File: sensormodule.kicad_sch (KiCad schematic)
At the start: 21 parts, among them X1 32.768KHz, X2 16MHz

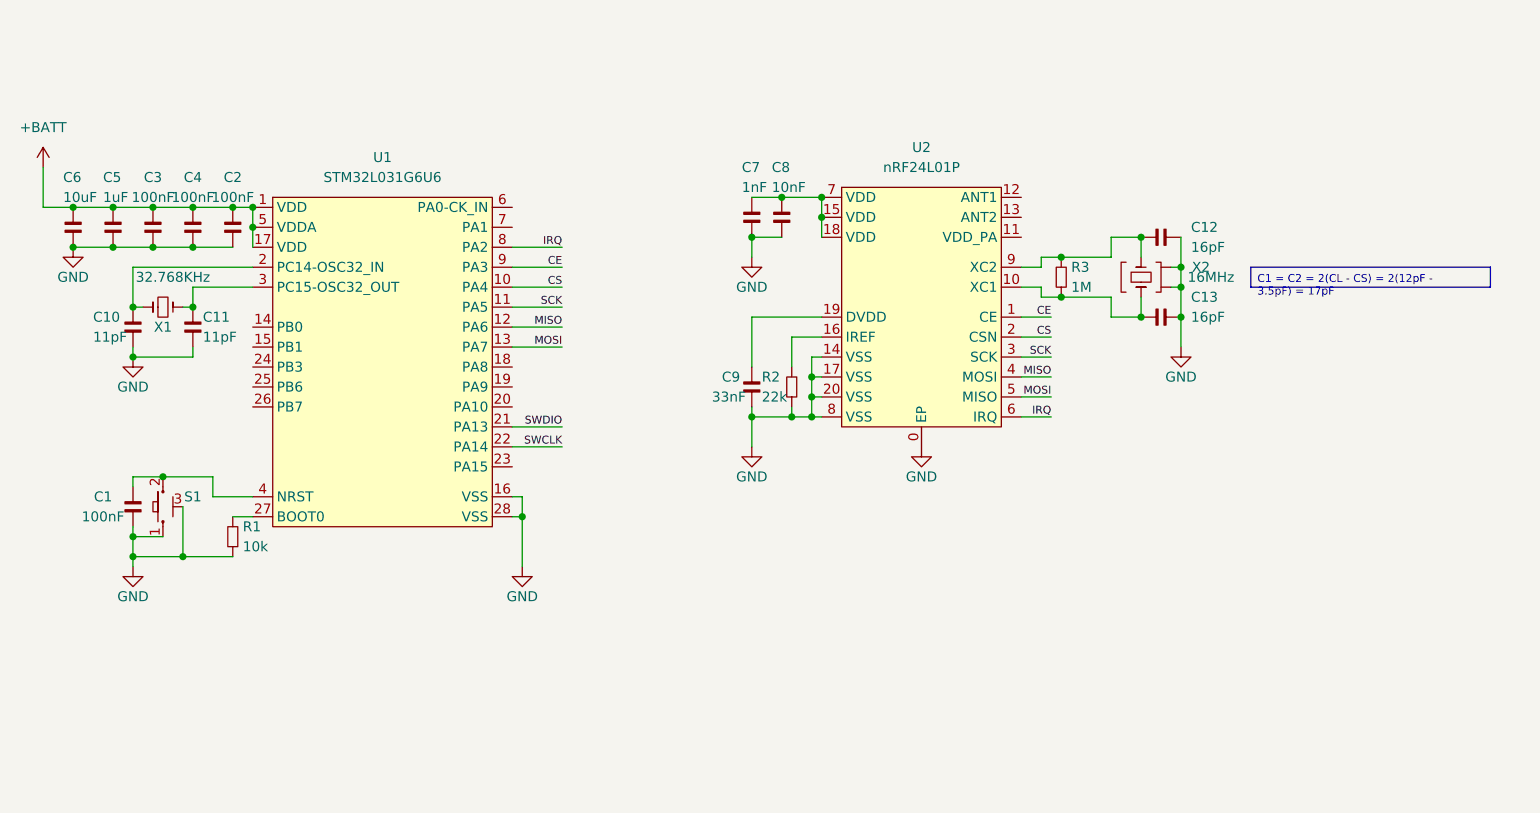
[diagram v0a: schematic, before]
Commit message: update
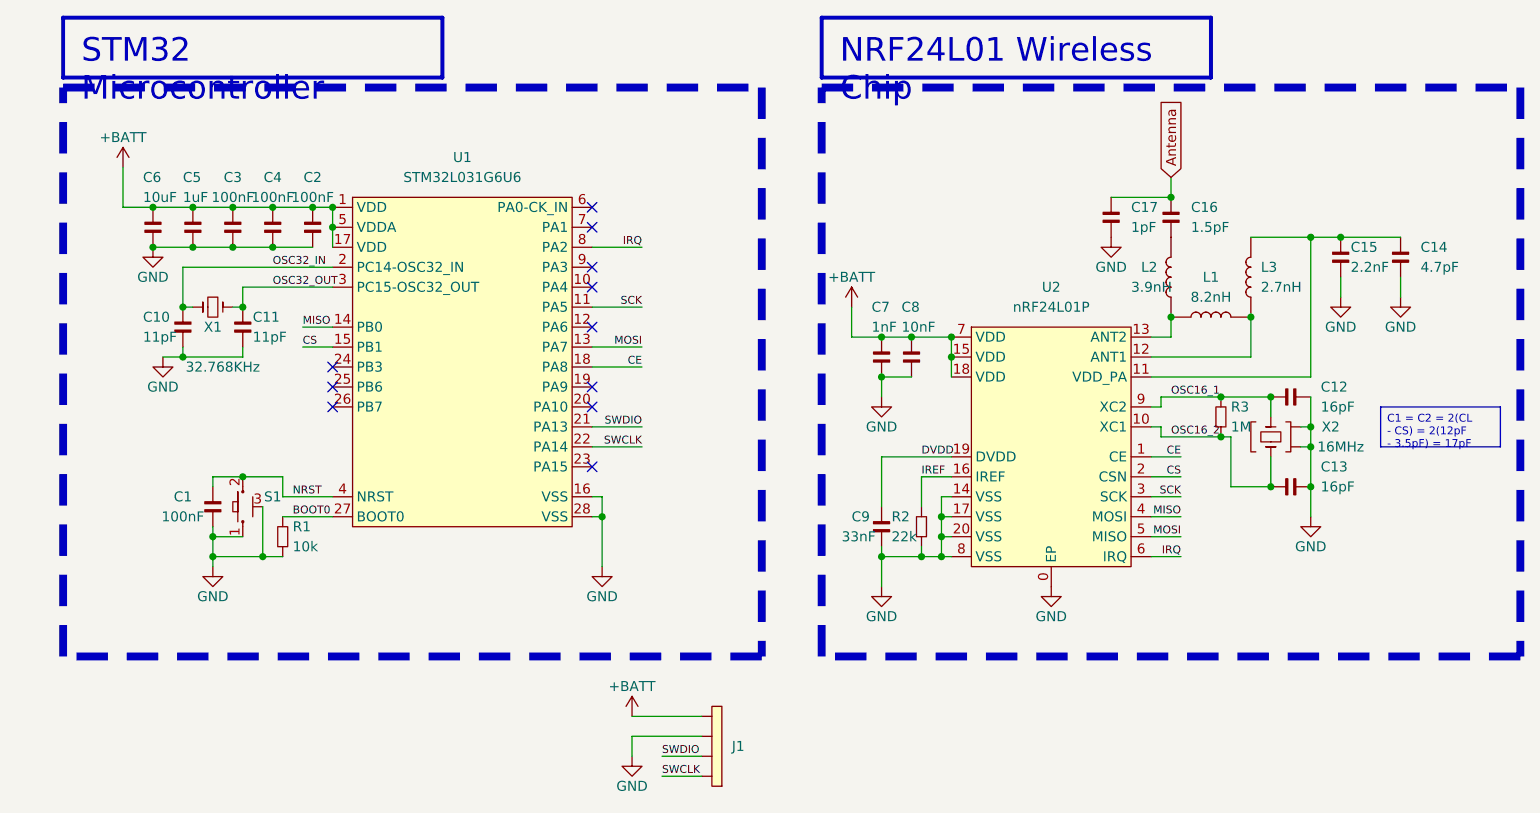
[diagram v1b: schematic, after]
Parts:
- added C14: 4.7pF, Kylian:[0402] Capacitor, symbol [0402] Kylian:[0402]_C_pF_4.7
- added C15: 2.2nF, Kylian:[0402] Capacitor, symbol [0402] Kylian:[0402]_C_nF_2.2
- added C16: 1.5pF, Kylian:[0402] Capacitor, symbol [0402] Kylian:[0402]_C_pF_1.5
- added C17: 1pF, Kylian:[0402] Capacitor, symbol [0402] Kylian:[0402]_C_pF_1
- added J1: [Header]_4-Pos_1.27mm, Kylian:[Header] 1.27mm 4-Position, symbol Kylian:[Header]_4-Pos_1.27mm
- added L1: 8.2nH, Kylian:[0402] Inductor, symbol [0402] Kylian:[0402]_L_nH_8.2
- added L2: 3.9nH, Kylian:[0402] Inductor, symbol [0402] Kylian:[0402]_L_nH_3.9
- added L3: 2.7nH, Kylian:[0402] Inductor, symbol [0402] Kylian:[0402]_L_nH_2.7
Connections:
- net +BATT: now also C7.2, C8.2, U2.15 (VDD), U2.18 (VDD), U2.7 (VDD), J1.4
- net CE: now also U1.18 (PA8); no longer U1.9 (PA3)
- net CS: now also U1.15 (PB1); no longer U1.10 (PA4)
- net GND: now also C14.1, C15.1, C17.1, J1.3
- net MISO: now also U1.14 (PB0); no longer U1.12 (PA6)
- net SWCLK: now also J1.1
- net SWDIO: now also J1.2
- net OSC16_2: now reaches C13.2, R3.1, U2.10 (XC1), X2.1
- net at U2.11 (VDD_PA): now also C14.2, C15.2, L3.2
- net at U2.12 (ANT1): now also L1.2, L3.1
- net at U2.13 (ANT2): now also L1.1, L2.1
- net IREF: now reaches R2.2, U2.16 (IREF)
- net DVDD: now reaches C9.2, U2.19 (DVDD)
- net OSC16_1: now reaches C12.2, R3.2, U2.9 (XC2), X2.3
- net OSC32_OUT: now reaches C11.2, U1.3 (PC15-OSC32_OUT), X1.2
- net NRST: now reaches C1.2, S1.2, U1.4 (NRST)
- net OSC32_IN: now reaches C10.2, U1.2 (PC14-OSC32_IN), X1.1
- net BOOT0: now reaches R1.2, U1.27 (BOOT0)
- new net: C16.1, L2.2
- new net Antenna: C16.2, C17.2
- no-connect marks 0 -> 11
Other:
- moved on the sheet: C1, C10, C11, C12, C13, C2, C3, C4, C5, C6, C7, C8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
